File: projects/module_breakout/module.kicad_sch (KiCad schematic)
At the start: 4 parts, among them J1 Conn_01x20_Pin, J2 Conn_01x20_Pin, J3 Conn_01x20_Pin, J4 Conn_01x20_Pin

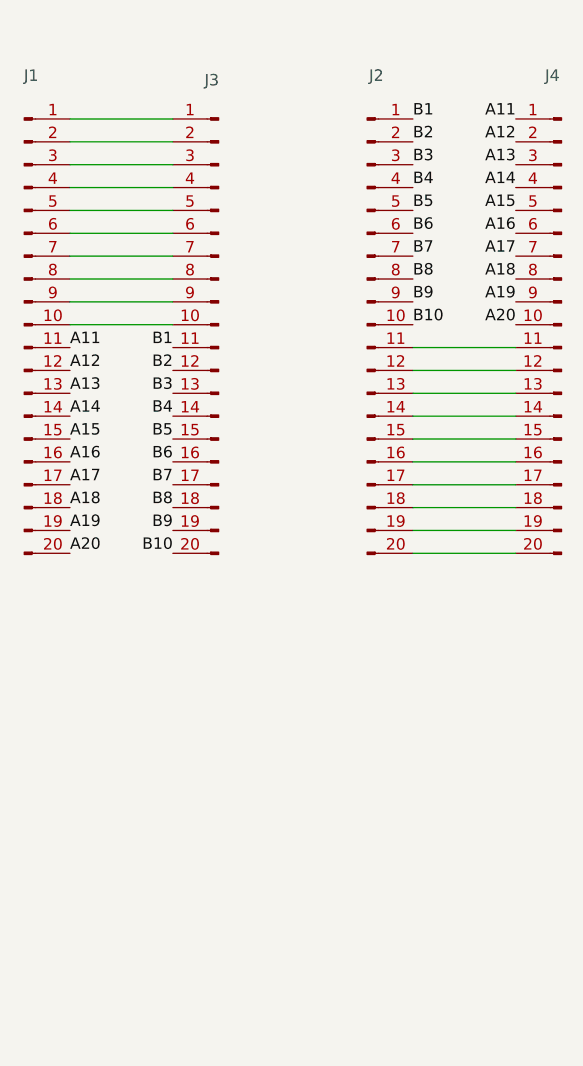
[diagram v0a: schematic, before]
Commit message: RF module test 4
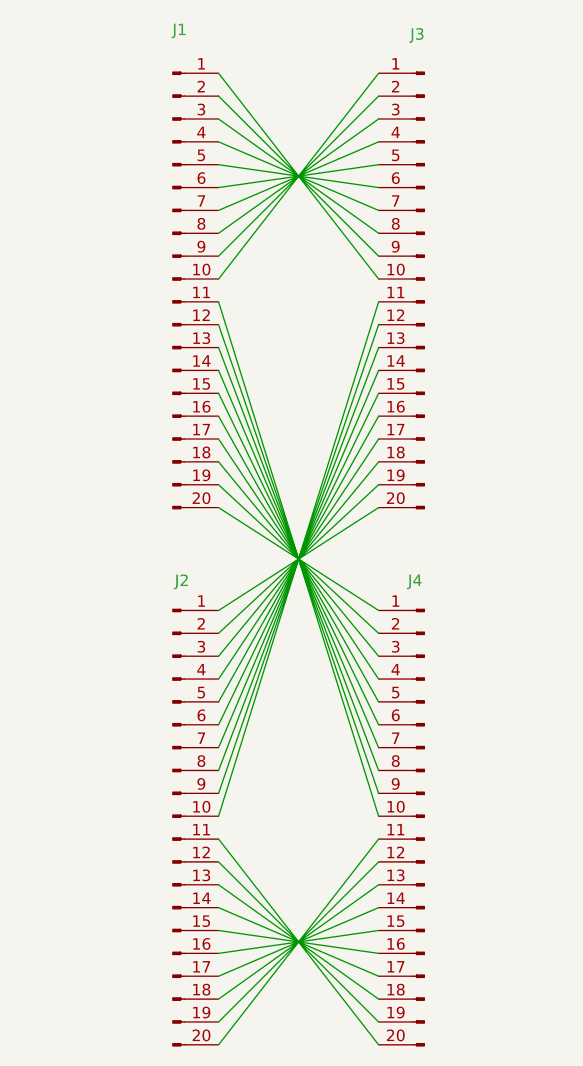
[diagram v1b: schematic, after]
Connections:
- net at J3.1 (Pin_1): now also J1.10 (Pin_10); no longer J1.1 (Pin_1)
- net at J3.10 (Pin_10): now also J1.1 (Pin_1); no longer J1.10 (Pin_10)
- net at J3.2 (Pin_2): now also J1.9 (Pin_9); no longer J1.2 (Pin_2)
- net at J3.3 (Pin_3): now also J1.8 (Pin_8); no longer J1.3 (Pin_3)
- net at J3.4 (Pin_4): now also J1.7 (Pin_7); no longer J1.4 (Pin_4)
- net at J3.5 (Pin_5): now also J1.6 (Pin_6); no longer J1.5 (Pin_5)
- net at J3.6 (Pin_6): now also J1.5 (Pin_5); no longer J1.6 (Pin_6)
- net at J3.7 (Pin_7): now also J1.4 (Pin_4); no longer J1.7 (Pin_7)
- net at J3.8 (Pin_8): now also J1.3 (Pin_3); no longer J1.8 (Pin_8)
- net at J3.9 (Pin_9): now also J1.2 (Pin_2); no longer J1.9 (Pin_9)
- net at J2.11 (Pin_11): now also J4.20 (Pin_20); no longer J4.11 (Pin_11)
- net at J2.12 (Pin_12): now also J4.19 (Pin_19); no longer J4.12 (Pin_12)
- net at J2.13 (Pin_13): now also J4.18 (Pin_18); no longer J4.13 (Pin_13)
- net at J2.14 (Pin_14): now also J4.17 (Pin_17); no longer J4.14 (Pin_14)
- net at J2.15 (Pin_15): now also J4.16 (Pin_16); no longer J4.15 (Pin_15)
- net at J2.16 (Pin_16): now also J4.15 (Pin_15); no longer J4.16 (Pin_16)
- net at J2.17 (Pin_17): now also J4.14 (Pin_14); no longer J4.17 (Pin_17)
- net at J2.18 (Pin_18): now also J4.13 (Pin_13); no longer J4.18 (Pin_18)
- net at J2.19 (Pin_19): now also J4.12 (Pin_12); no longer J4.19 (Pin_19)
- net at J2.20 (Pin_20): now also J4.11 (Pin_11); no longer J4.20 (Pin_20)
- net A11: no longer names the net of J1.11 (Pin_11)
- net A11: now also J4.10 (Pin_10); no longer J4.1 (Pin_1)
- net A12: no longer names the net of J1.12 (Pin_12)
- net A12: now also J4.9 (Pin_9); no longer J4.2 (Pin_2)
- net A13: no longer names the net of J1.13 (Pin_13)
- net A13: now also J4.8 (Pin_8); no longer J4.3 (Pin_3)
- net A14: no longer names the net of J1.14 (Pin_14)
- net A14: now also J4.7 (Pin_7); no longer J4.4 (Pin_4)
- net A15: no longer names the net of J1.15 (Pin_15)
- net A15: now also J4.6 (Pin_6); no longer J4.5 (Pin_5)
- net A16: no longer names the net of J1.16 (Pin_16)
- net A16: now also J4.5 (Pin_5); no longer J4.6 (Pin_6)
- net A17: no longer names the net of J1.17 (Pin_17)
- net A17: now also J4.4 (Pin_4); no longer J4.7 (Pin_7)
- net A18: no longer names the net of J1.18 (Pin_18)
- net A18: now also J4.3 (Pin_3); no longer J4.8 (Pin_8)
- net A19: no longer names the net of J1.19 (Pin_19)
- net A19: now also J4.2 (Pin_2); no longer J4.9 (Pin_9)
- net A20: no longer names the net of J1.20 (Pin_20)
- net A20: now also J4.1 (Pin_1); no longer J4.10 (Pin_10)
- net B1: no longer names the net of J3.11 (Pin_11)
- net B1: now also J2.10 (Pin_10); no longer J2.1 (Pin_1)
- net B10: no longer names the net of J3.20 (Pin_20)
- net B10: now also J2.1 (Pin_1); no longer J2.10 (Pin_10)
- net B2: no longer names the net of J3.12 (Pin_12)
- net B2: now also J2.9 (Pin_9); no longer J2.2 (Pin_2)
- net B3: no longer names the net of J3.13 (Pin_13)
- net B3: now also J2.8 (Pin_8); no longer J2.3 (Pin_3)
- net B4: no longer names the net of J3.14 (Pin_14)
- net B4: now also J2.7 (Pin_7); no longer J2.4 (Pin_4)
- net B5: no longer names the net of J3.15 (Pin_15)
- net B5: now also J2.6 (Pin_6); no longer J2.5 (Pin_5)
- net B6: no longer names the net of J3.16 (Pin_16)
- net B6: now also J2.5 (Pin_5); no longer J2.6 (Pin_6)
- net B7: no longer names the net of J3.17 (Pin_17)
- net B7: now also J2.4 (Pin_4); no longer J2.7 (Pin_7)
- net B8: no longer names the net of J3.18 (Pin_18)
- net B8: now also J2.3 (Pin_3); no longer J2.8 (Pin_8)
- net B9: no longer names the net of J3.19 (Pin_19)
- net B9: now also J2.2 (Pin_2); no longer J2.9 (Pin_9)
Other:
- moved on the sheet: J1, J2, J3, J4
